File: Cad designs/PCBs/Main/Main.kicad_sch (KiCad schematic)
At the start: 4 parts, among them J1 Power, J2 Digital/PWM, J3 Analog, J4 Digital/PWM

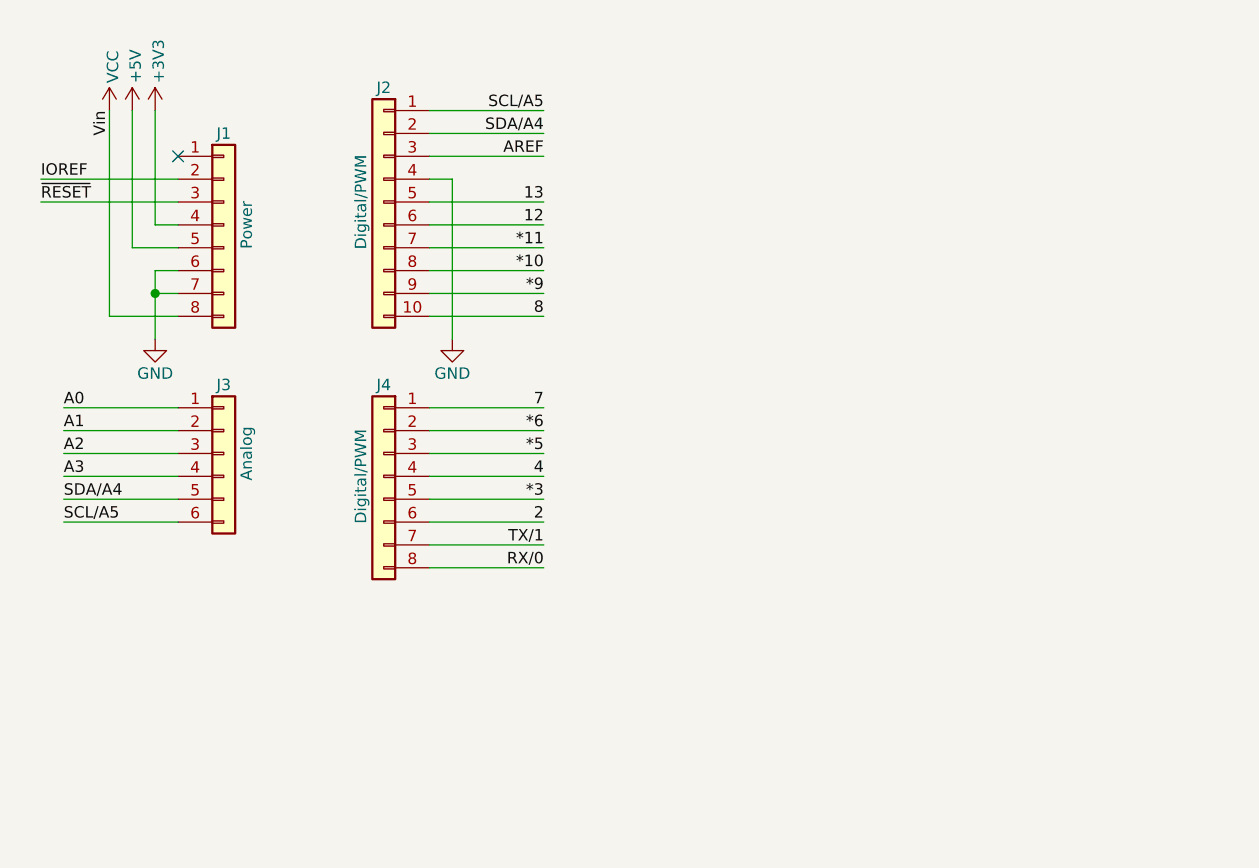
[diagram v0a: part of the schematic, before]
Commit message: 12/08/26
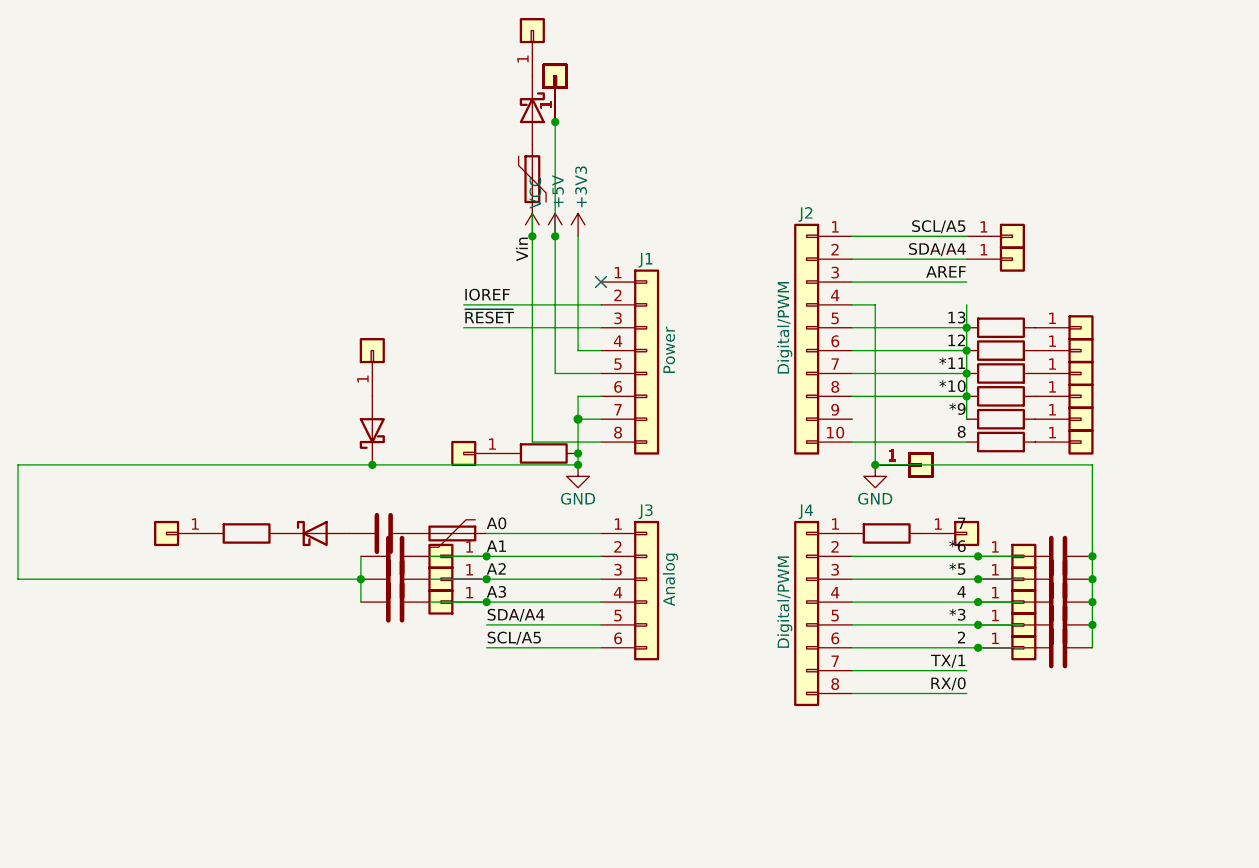
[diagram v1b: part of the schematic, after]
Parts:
- added C1, C2, C3, C4, C5, C6, C7, C8, C9: C, Capacitor_THT:C_Disc_D5.0mm_W2.5mm_P2.50mm, symbol Device:C
- added D1, D2, D3: 1N5819, Diode_THT:D_DO-201AD_P15.24mm_Horizontal, symbol Diode:1N5819
- added F1, F2: Polyfuse, Fuse:Fuse_Bourns_MF-RHT050, symbol Device:Polyfuse
- added J10, J11, J12, J13, J14, J15, J16, J17, J18, J19, J20, J21, J22, J23, J24, J25, J26, J27, J28, J29, J30, J31, J32, J33, J34, J35, J36, J37, J38, J39, J40, J41, J42, J43, J44, J45, J46, J47, J48, J49, J5, J50, J6, J7, J8, J9: Conn_01x01, Connector_Wire:SolderWire-0.127sqmm_1x01_D0.48mm_OD1mm, symbol Connector_Generic:Conn_01x01
- added R1, R2, R3, R4, R5, R6, R7, R8, R9: R, Resistor_THT:R_Axial_DIN0207_L6.3mm_D2.5mm_P7.62mm_Horizontal, symbol Device:R
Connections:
- net *11 is gone; now on net *10: J2.7 (Pin_7)
- net 12 is gone; now on net *10: J2.6 (Pin_6)
- net 13 is gone; now on net *10: J2.5 (Pin_5)
- net *10: now also R3.1, R4.1, R5.1, R6.1, R7.2
- net *3: now also C8.1, J42.1 (Pin_1)
- net *5: now also C3.1, J40.1 (Pin_1)
- net *6: now also C4.1, J39.1 (Pin_1)
- net +5V: now also J22.1 (Pin_1), J23.1 (Pin_1), J27.1 (Pin_1), J28.1 (Pin_1), J29.1 (Pin_1), J33.1 (Pin_1), J34.1 (Pin_1), J35.1 (Pin_1), J36.1 (Pin_1)
- net 2: now also C5.1, J43.1 (Pin_1)
- net 4: now also C7.1, J41.1 (Pin_1)
- net 7: no longer J4.1 (Pin_1)
- net 8: now also R2.1
- net A0: now also F2.1
- net A1: now also C9.1, J44.1 (Pin_1)
- net A2: now also C6.1, J45.1 (Pin_1)
- net A3: now also C2.1, J46.1 (Pin_1)
- net GND: now also C2.2, C3.2, C4.2, C5.2, C6.2, C7.2, C8.2, C9.2, D3.1 (K), J11.1 (Pin_1), J12.1 (Pin_1), J13.1 (Pin_1), J14.1 (Pin_1), J15.1 (Pin_1), J16.1 (Pin_1), J17.1 (Pin_1), J18.1 (Pin_1), J19.1 (Pin_1), J20.1 (Pin_1), J21.1 (Pin_1), J5.1 (Pin_1), J6.1 (Pin_1), J7.1 (Pin_1), J8.1 (Pin_1), J9.1 (Pin_1), R9.1
- net SCL/A5: now also J10.1 (Pin_1)
- net SDA/A4: now also J31.1 (Pin_1)
- net VCC: now also F1.2
- net *9: no longer names the net of J2.9 (Pin_9)
- new net: J4.1 (Pin_1), R1.2
- new net: D1.1 (K), R8.1
- new net: C1.2, D1.2 (A)
- new net: J30.1 (Pin_1), R4.2
- new net: J24.1 (Pin_1), R2.2
- new net: J25.1 (Pin_1), R3.2
- new net: J49.1 (Pin_1), R9.2
- new net: D2.1 (K), J47.1 (Pin_1)
- new net: D2.2 (A), F1.1
- new net: J48.1 (Pin_1), R8.2
- new net: J32.1 (Pin_1), R1.1
- new net: D3.2 (A), J50.1 (Pin_1)
- new net: J26.1 (Pin_1), R6.2
- new net: C1.1, F2.2
- new net: J37.1 (Pin_1), R7.1
- new net: J38.1 (Pin_1), R5.2
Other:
- moved on the sheet: J1, J2, J3, J4
